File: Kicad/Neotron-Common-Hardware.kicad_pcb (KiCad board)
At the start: 4 copper layers, 243.8 x 243.8 mm, 319 parts, among them J1001 RJ45 MagJack, J101 Neotron-Expansion-Slot, J102 Neotron-Expansion-Slot, J103 Neotron-Expansion-Slot, J104 Neotron-Expansion-Slot, J1201 DE15HD, J1601 Header, J1602 Header, J1603 Conn_01x05, J1604 Double-mini-DIN-6, J1701 Jack 2/6.3mm, J201 DE15HD, J601 CD Audio In, J602 AC'97 Audio Header, J603 Line Out, J701 SD_Card, J801 Conn_02x05, J802 DB9_Male_MountingHoles, J901 USB Ports External, J902 USB Ports Internal, Q1701 BC546, Q1702 BC556, SW1601 SW_DIP_x01, SW1602 SW_DIP_x01, U1001 ENC424J600, U101 Neotron-CPU, U1101 MCP7940N, U1201 THS7316, U1202 TPD7S019, U1601 STM32F031K6T6, U1701 DC-DC Module, U1702 MAX1615, U1703 TLV1117 3.3V 1A, U1801 MCP23S17_SO, U1802 74HC245, U201 THS7316, U202 TPD7S019, U601 TLV320AIC23BPW, U602 STX-4335-5BGP-S1, U801 ST3232CDR, U901 AP2501, U902 XR22404CG28, U903 MIC2005A-2YM5, U904 MIC2005A-2YM5, U905 MIC2005A-2YM5, U906 MIC2005A-2YM5, Y1001 25M, Y1101 32,768 Hz, Y601 12M 20pF, Y901 12M

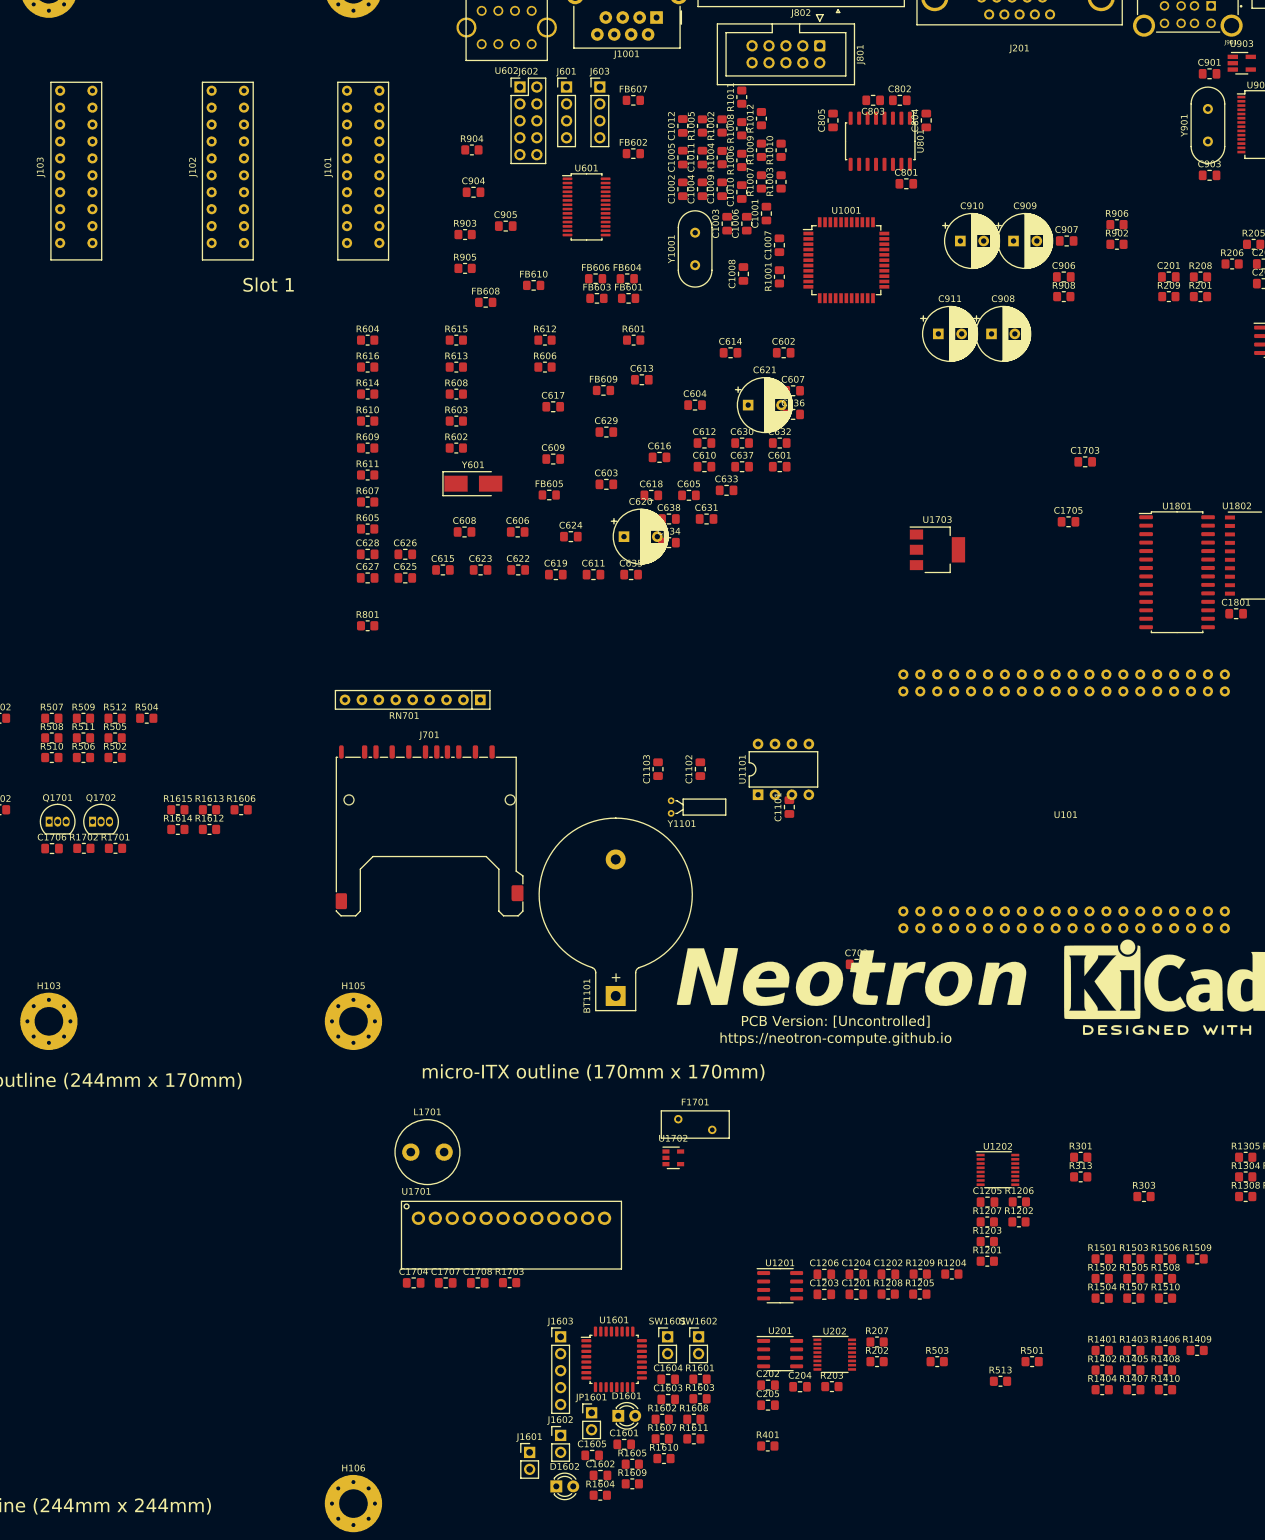
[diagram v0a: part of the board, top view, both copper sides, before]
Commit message: Update fileformats to Kicad 6.
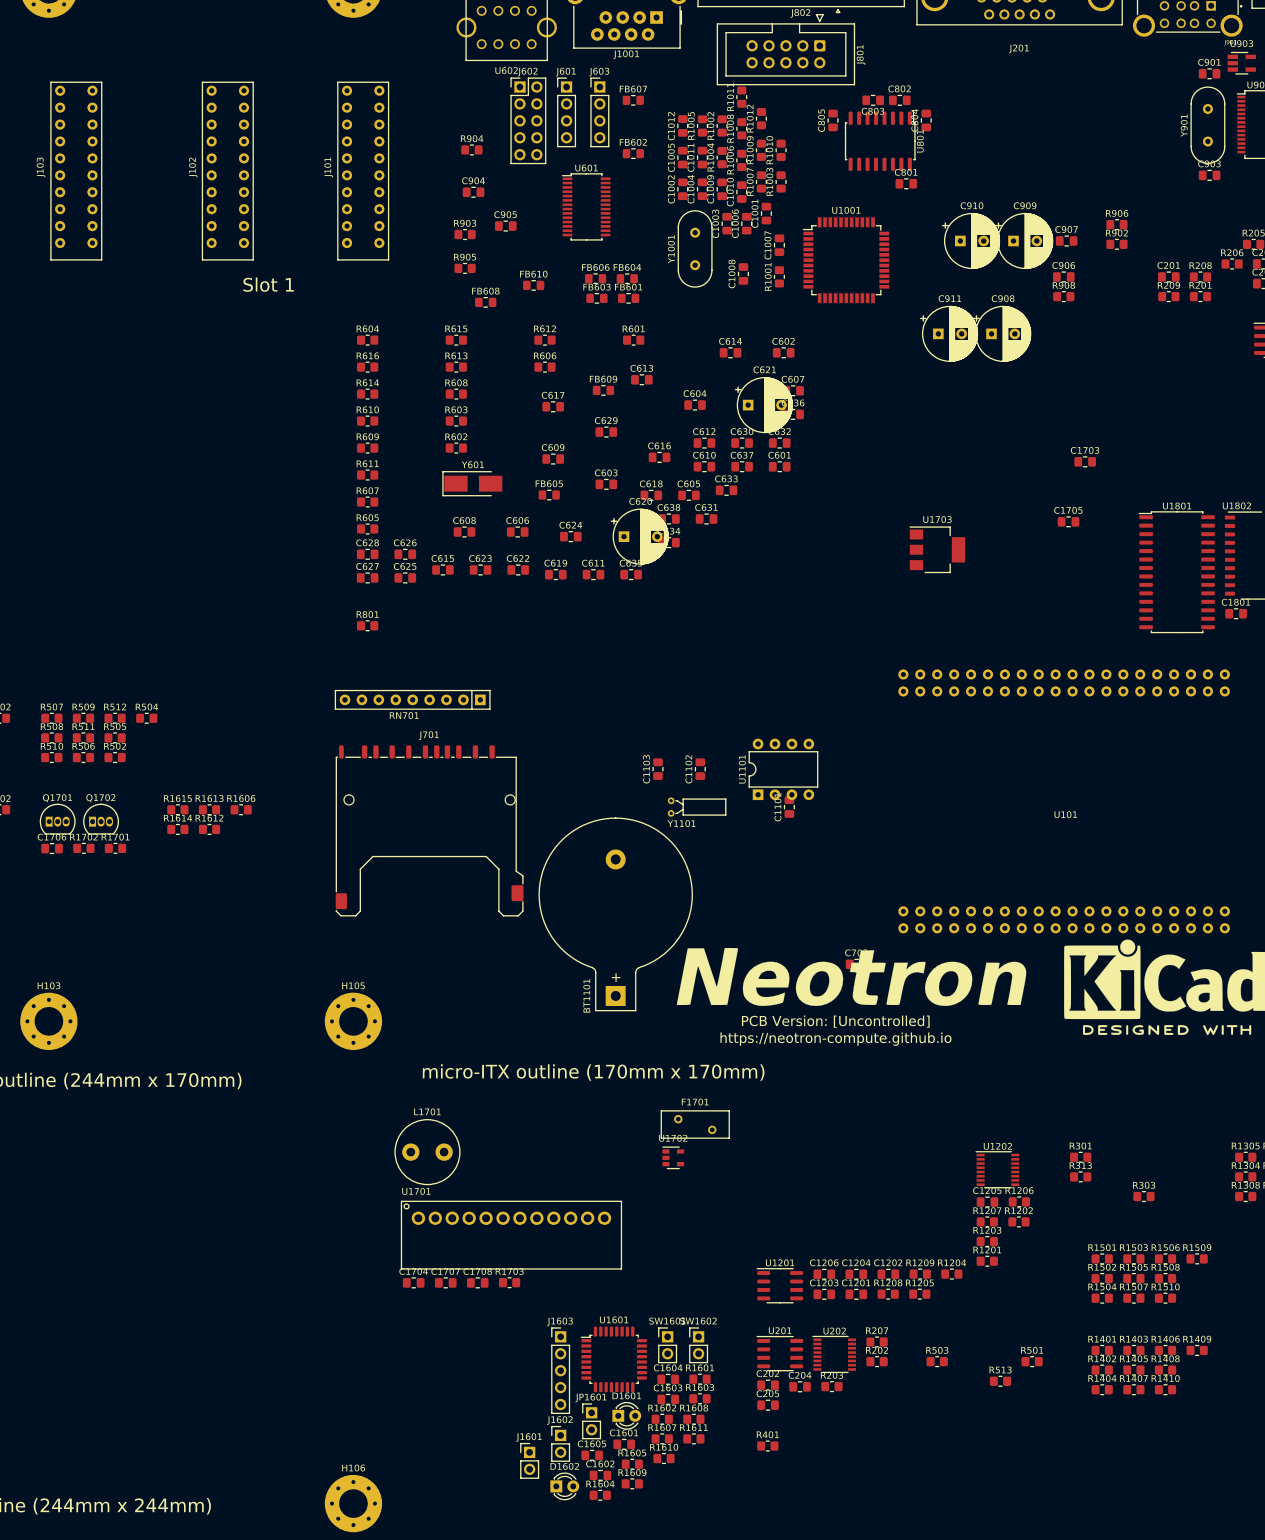
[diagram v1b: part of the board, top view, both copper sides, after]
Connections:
- net /Board Management Controller/~BMC_RST renamed /Board Management Controller/~{BMC_RST}
- net /Board Management Controller/~BUTTON_PWR renamed /Board Management Controller/~{BUTTON_PWR}
- net /Board Management Controller/~BUTTON_RST renamed /Board Management Controller/~{BUTTON_RST}
- net /Board Management Controller/~RESET renamed /Board Management Controller/~{RESET}
- net /Ethernet/~IRQ renamed /Ethernet/~{IRQ}
- net /IO Expander/~CS0 renamed /IO Expander/~{CS0}
- net /IO Expander/~CS1 renamed /IO Expander/~{CS1}
- net /IO Expander/~CS2 renamed /IO Expander/~{CS2}
- net /IO Expander/~CS3 renamed /IO Expander/~{CS3}
- net /IO Expander/~CS4 renamed /IO Expander/~{CS4}
- net /IO Expander/~CS5 renamed /IO Expander/~{CS5}
- net /IO Expander/~CS6 renamed /IO Expander/~{CS6}
- net /IO Expander/~CS7 renamed /IO Expander/~{CS7}
- net /Power Supply and BMC/~SHDN renamed /Power Supply and BMC/~{SHDN}
- net /SD Card/~CARD_DETECT renamed /SD Card/~{CARD_DETECT}
- net /SD Card/~WRITE_PROTECT renamed /SD Card/~{WRITE_PROTECT}
- net /USB/~ENABLE renamed /USB/~{ENABLE}
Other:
- net class Default removed
